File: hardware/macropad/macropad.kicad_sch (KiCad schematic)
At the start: 35 parts, among them J1 SWD, J2 USB_C_Receptacle_USB2.0_16P, J3 Conn_01x02, J4 display(4x1), J6 Enc2, J7 Enc1, SW1 SW_Push, SW12 RotaryEncoder_Switch, SW13 RotaryEncoder_Switch, SW2 SW_Push, SW3 SW_Push, SW4 SW_Push, SW5 SW_Push, SW6 SW_Push, SW7 SW_Push, SW8 SW_Push, SW9 SW_Push, U2 STM32F103C8Tx, U3 NRF24L01_Breakout, Y1 8Mhz C_L=12pF

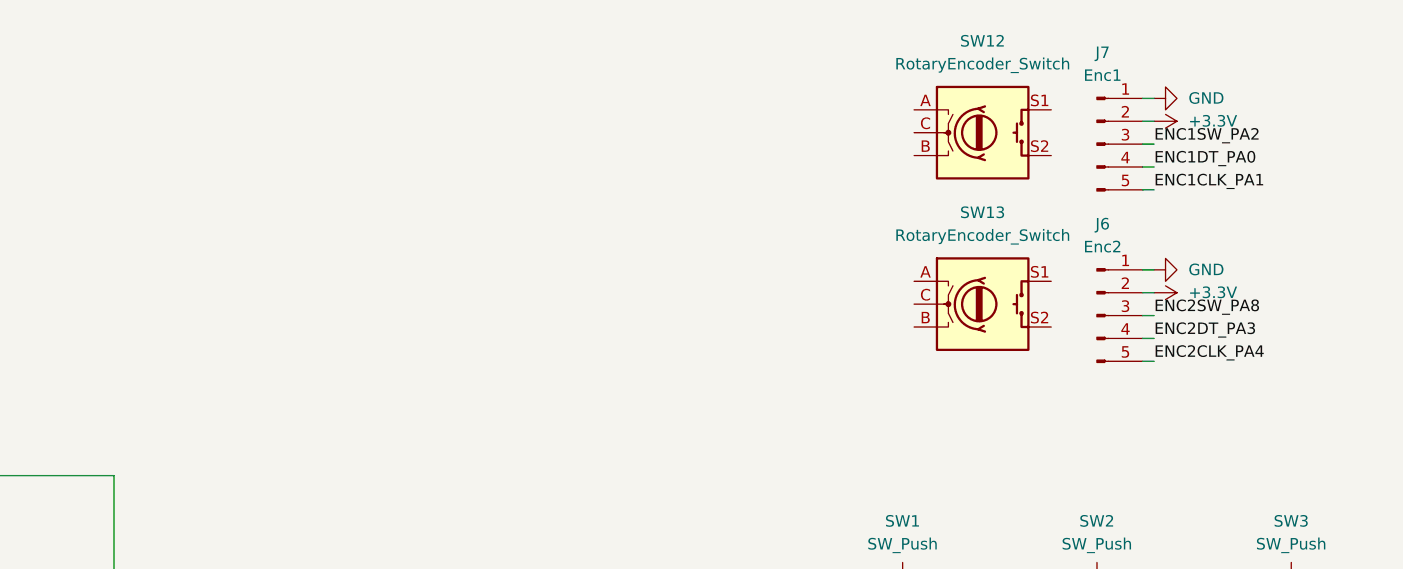
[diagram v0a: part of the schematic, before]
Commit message: pcb done
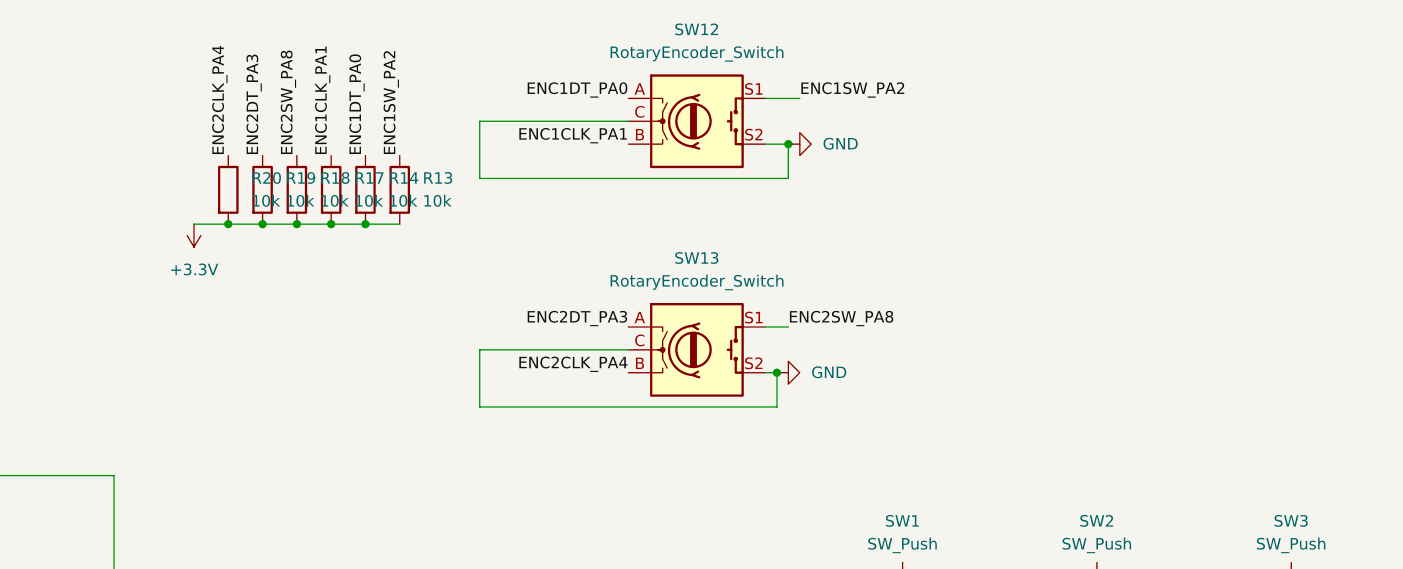
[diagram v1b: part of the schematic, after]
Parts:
- removed J6: Enc2, Connector_PinHeader_2.54mm:PinHeader_1x05_P2.54mm_Vertical, symbol Connector:Conn_01x05_Pin
- removed J7: Enc1, Connector_PinHeader_2.54mm:PinHeader_1x05_P2.54mm_Vertical, symbol Connector:Conn_01x05_Pin
- added R13, R14, R17, R18, R19, R20: 10k, Resistor_SMD:R_0805_2012Metric, symbol Device:R
- SW12, SW13: footprint (none) -> Rotary_Encoder:RotaryEncoder_Alps_EC12E-Switch_Vertical_H20mm
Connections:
- net +3.3V: now also R13.2, R14.2, R17.2, R18.2, R19.2, R20.2
- net ENC1CLK_PA1: now also SW12.B, R17.1
- net ENC1DT_PA0: now also SW12.A, R14.1
- net ENC1SW_PA2: now also SW12.S1, R13.1
- net ENC2CLK_PA4: now also SW13.B, R20.1
- net ENC2DT_PA3: now also SW13.A, R19.1
- net ENC2SW_PA8: now also SW13.S1, R18.1
- net GND: now also SW12.C, SW12.S2, SW13.C, SW13.S2
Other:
- moved on the sheet: SW12, SW13
